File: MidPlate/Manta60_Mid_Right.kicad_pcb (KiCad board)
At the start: 2 copper layers, 168.9 x 121.4 mm, 104 parts, among them P1 LED-pin, SW1 SW_Push, SW10 SW_Push, SW11 SW_Push, SW12 SW_Push, SW13 SW_Push, SW14 SW_Push, SW15 SW_Push, SW16 SW_Push, SW17 SW_Push, SW18 SW_Push, SW19 SW_Push, SW2 SW_Push, SW20 SW_Push, SW21 SW_Push, SW22 SW_Push, SW23 SW_Push, SW24 SW_Push, SW25 SW_Push, SW26 SW_Push, SW27 SW_Push, SW28 SW_Push, SW29 SW_Push, SW3 SW_Push, SW30 SW_Push, SW31 SW_Push, SW32 SW_Push, SW33 SW_Push, SW34 SW_Push, SW35 SW_Push, SW4 SW_Push, SW5 SW_Push, SW6 SW_Push, SW7 SW_Push, SW8 SW_Push, SW9 SW_Push, T1 TRRS, U1 ProMicro

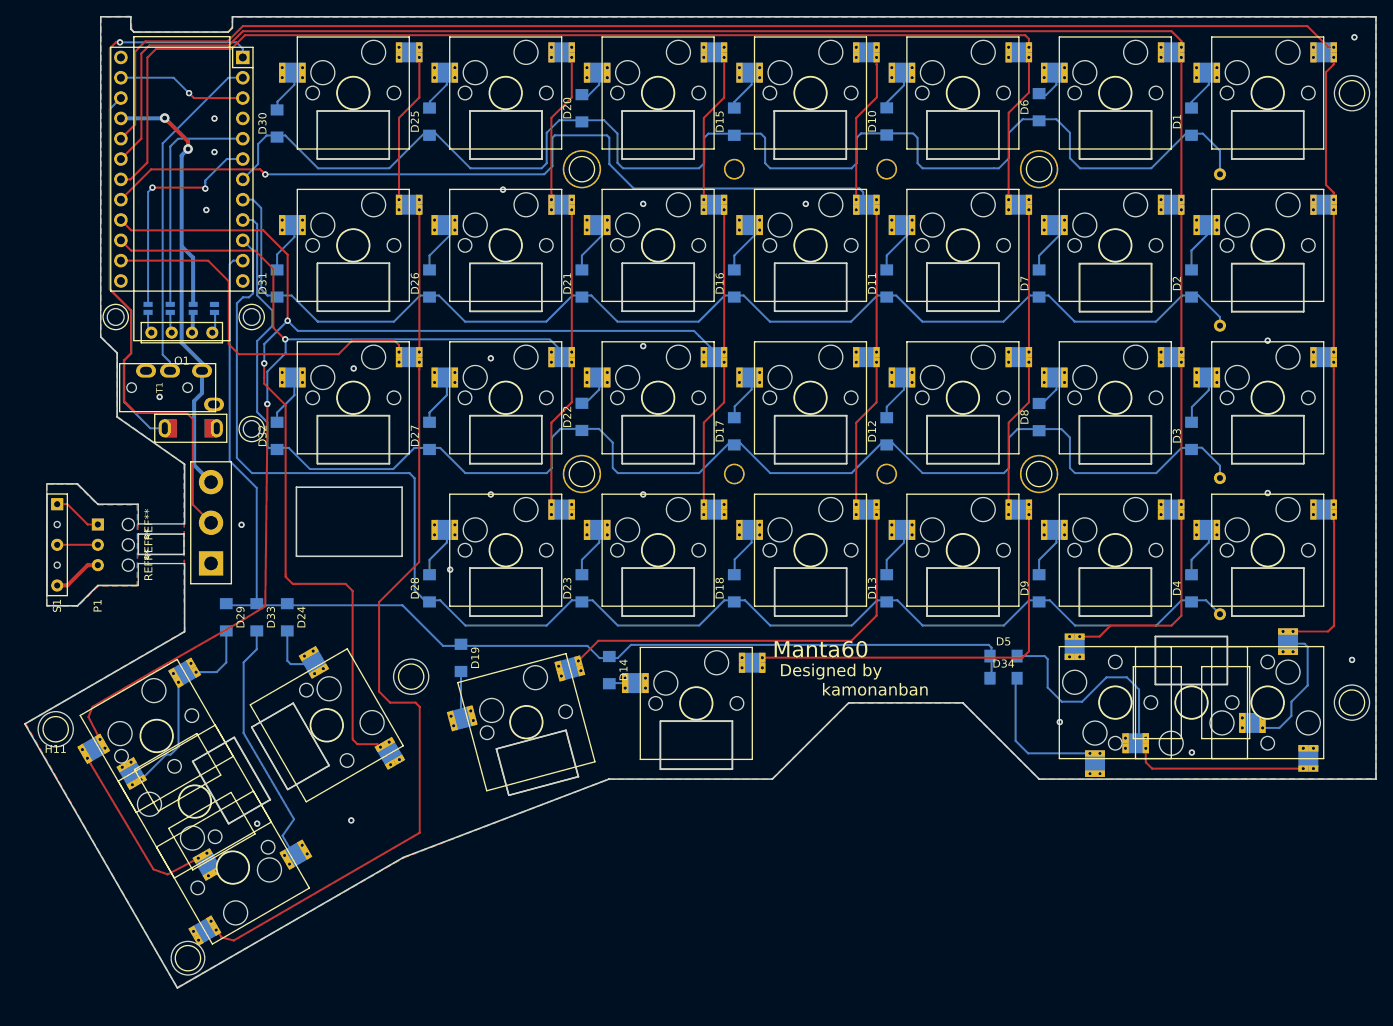
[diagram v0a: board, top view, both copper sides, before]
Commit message: update
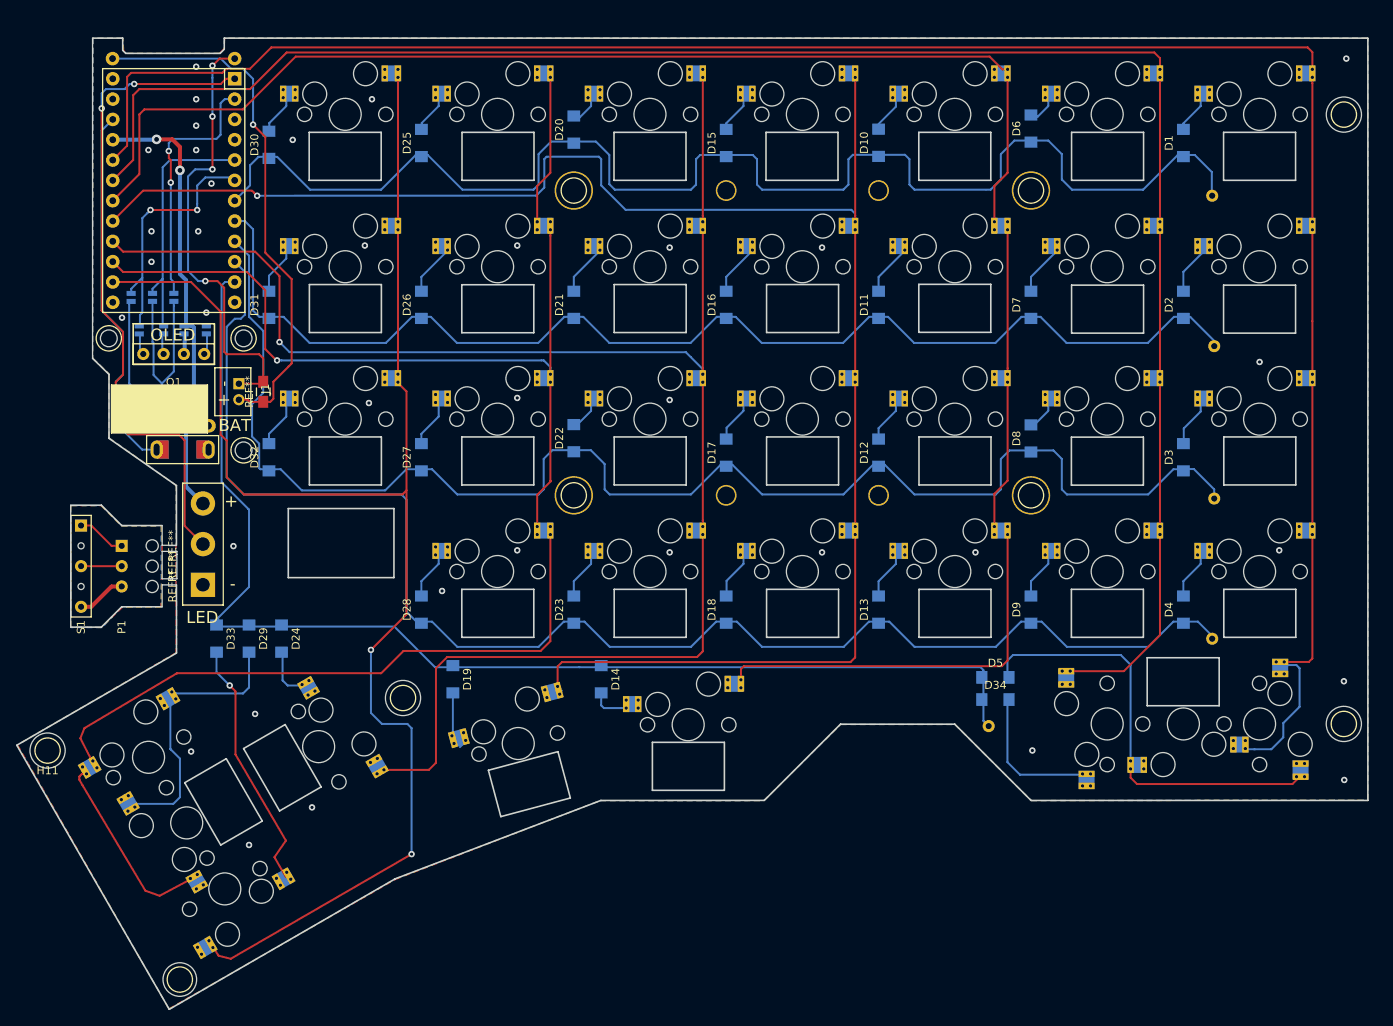
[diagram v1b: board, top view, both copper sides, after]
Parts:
- removed JP8: SolderJumper, library:Jumper3
- added ?: , library:GND, F.Cu at (184.1, 128.5)
- added J1: Conn_01x02, manta60:PH_2Pin_Top, F.Cu at (90.4, 86.7)
- added JP1: , library:Jumper3, B.Cu at (86.3, 79.0)
- added JP2: , library:Jumper3, B.Cu at (83.5, 79.0)
- added JP3: , library:Jumper3, B.Cu at (81.0, 79.0)
- added JP4: , library:Jumper3, B.Cu at (77.9, 79.0)
- added REF**: C_0805, Capacitors_SMD:C_0805_HandSoldering, F.Cu at (93.4, 86.7)
- H8: value HOLE -> (none)
- JP5, JP6, JP7: value SolderJumper -> (none)
- O1: footprint library:OLED -> manta60:OLED
- SW1, SW10, SW11, SW12, SW13, SW14, SW15, SW16, SW17, SW18, SW19, SW2, SW20, SW21, SW22, SW23, SW24, SW25, SW26, SW27, SW28, SW3, SW30, SW31, SW32, SW33, SW35, SW4, SW6, SW7, SW8, SW9: footprint manta60:Kailh-socket_re -> manta60:CherryMX_Hotswap_right
- SW29 (x2), SW5 (x2): footprint manta60:Kailh-socket -> manta60:CherryMX_Hotswap_left
- SW34: value SW_Push -> Reset_SW
- U1: footprint library:ProMicro -> manta60:ProMicro
- moved D33 5.70 mm to (87.6, 117.6)
- moved JP6 5.08 mm to (76.9, 74.9)
- moved P1 4.00 mm to (75.7, 108.5)
- moved REF** 4.00 mm to (79.6, 106.0)
- moved REF** 4.00 mm to (79.6, 108.5)
- moved REF** 4.00 mm to (79.6, 111.1)
- moved S1 4.00 mm to (70.7, 108.5)
- moved D29 3.90 mm to (91.7, 117.6)
- moved ? 3.22 mm to (212.1, 117.6)
- moved ? 2.86 mm to (212.1, 62.2)
- moved D1 2.85 mm to (208.5, 55.6)
- moved D15 2.85 mm to (151.3, 55.6)
- moved D16 2.85 mm to (151.3, 75.9)
- moved D17 2.85 mm to (151.3, 94.3)
- moved D2 2.85 mm to (208.5, 75.9)
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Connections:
- JP5 pad 1: Net-(JP4-Pad1) -> Net-(JP5-Pad1)
- JP5 pad 2: SDA -> SCL
- JP6 pad 1: Net-(JP3-Pad1) -> Net-(JP6-Pad1)
- JP6 pad 2: SCL -> SDA
- JP7 pad 1: Net-(JP2-Pad1) -> Net-(JP5-Pad1)
- JP7 pad 2: VCC -> Data
- T1 pad B: Net-(T1-PadB) -> Net-(JP6-Pad1)
- T1 pad C: Data -> Net-(JP5-Pad1)
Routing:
- net BAT: track 0.00 -> 66.1 mm, vias 0 -> 1
- net BAT_GND: track 0.00 -> 56.6 mm, vias 0 -> 4
- net Col2: track 261.5 -> 230.7 mm
- net Col0: track 285.3 -> 256.9 mm
- net Col1: track 251.9 -> 223.8 mm
- net Col4: track 236.0 -> 208.1 mm, vias 2 -> 1
- net Net-(JP5-Pad1): track 0.00 -> 23.8 mm
- net Col3: track 239.0 -> 217.3 mm
- net GND: track 17.3 -> 1.53 mm, vias 23 -> 37
- net Col5: track 240.4 -> 224.7 mm, vias 2 -> 1
- net Net-(JP6-Pad1): track 0.00 -> 11.9 mm
- net Data: track 42.2 -> 32.0 mm, vias 0 -> 2
- net Col6: track 198.4 -> 189.9 mm, vias 0 -> 2
- net Net-(D5-Pad2): track 60.4 -> 53.1 mm
- net VCC: track 62.8 -> 55.8 mm
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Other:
- outline, holes or cut-outs redrawn
- board text added: "+"
- board text added: "-"
- board text added: "BAT"
- board text added: "C0"
- board text added: "C4"
- board text added: "Col0"
- board text added: "Col1"
- board text added: "Col2"
- board text added: "Col3"
- board text added: "Col4"
- board text added: "Col5"
- board text added: "Col6"
- board text added: "I2C"
- board text added: "LED"
- board text added: "OLED"
- board text added: "R0"
- board text added: "R4"
- board text added: "RX"
- board text added: "Row0"
- board text added: "Row1"
- board text added: "Row2"
- board text added: "Row3"
- board text added: "Row4"
